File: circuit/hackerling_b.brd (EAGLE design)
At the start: 82.5 x 67.4 mm, 45 parts, among them IC1 MCP23017SP, IC2 MCP2300X/P, IC3 MIC5219BM5, SW2 SWITCH_B13EH, U1 MMA8452Q, U2 LCD_16X2, U3 ARDUINOR3-BPLACE, U4 ACCELEROMETER, U5 PCA9306, U6 ACCELEROMETER, U7 POT, U8 SML_POT

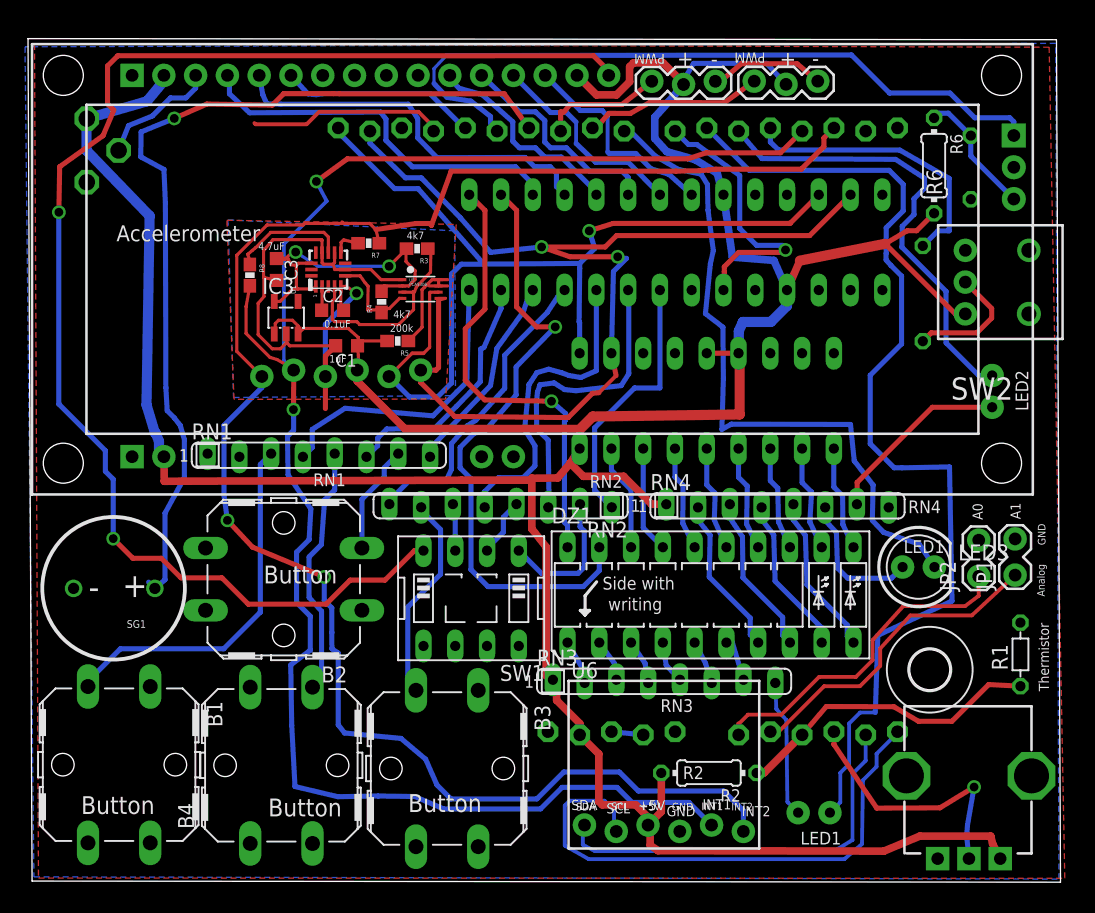
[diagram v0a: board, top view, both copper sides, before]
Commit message: changes made for version 1.2. ordered boards.
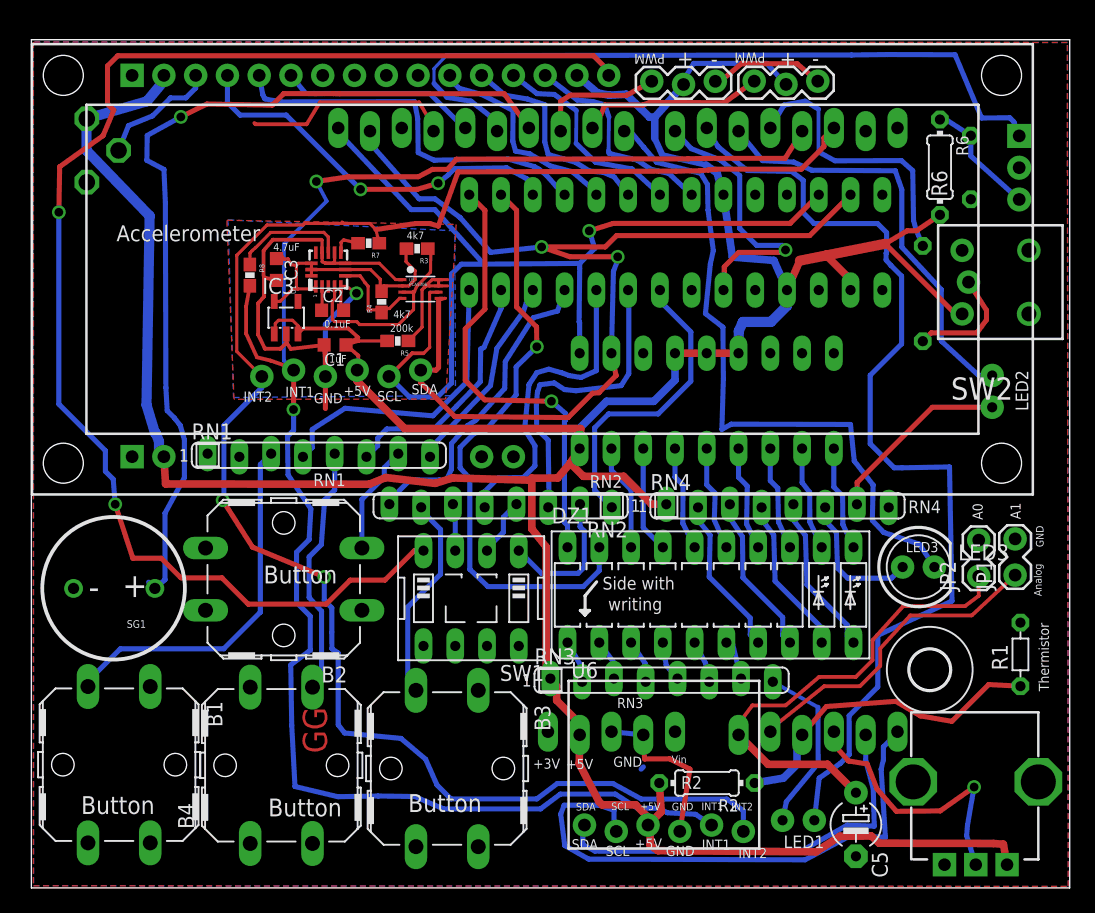
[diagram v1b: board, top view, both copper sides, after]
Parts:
- added C5: (no value), rcl:E5-4
- added U$2: HS-LOGOSMALL, hackerscouts:HS-LOGO-SM
- C4: device rcl:C050-050X075 -> hackerscouts:CAP_050X075
- moved LED1 1.39 mm to (61.3, 4.91)
- moved C1 0.92 mm to (24.3, 42.9)
- moved R2 0.82 mm to (54.0, 7.88)
- moved U7 0.73 mm to (75.5, 7.66)
- moved R6 0.49 mm to (72.6, 57.1)
- moved IR1 0.43 mm to (79.0, 57.1)
- moved RN3 0.22 mm to (50.4, 16.1)
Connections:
- net DIP1 renamed DIP4
- net DIPR1 renamed DIPR4
- net 3.3V: now also U1.15, U1.16, U1.7
- net DIP2: now also RN2.6, SW1.3; no longer RN2.4, SW1.2
- net DIP3: now also RN2.4, SW1.2; no longer RN2.6, SW1.3
- net DIPR2: now also IC1.24, RN2.5; no longer IC1.23, RN2.3
- net DIPR3: now also IC1.23, RN2.3; no longer IC1.24, RN2.5
- net GND: now also C5.-, U1.8; no longer IC1.16, IC2.4, U1.7
- net N$26: now also C5.+
- net VCC: now also IC1.16, IC2.4
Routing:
- net GND: track 75.1 -> 86.9 mm
- net N$26: track 26.8 -> 38.1 mm
- net 3.3V: track 26.6 -> 22.9 mm, vias 2 -> 0
- net DIPR4: track 21.3 -> 24.5 mm
- net N$32: track 11.0 -> 14.1 mm
- net IR_OUT2: track 36.4 -> 33.9 mm
- net BARGRAPH1: track 49.6 -> 47.5 mm
- net IR_OUT1: track 81.2 -> 79.1 mm
- net TEMP: track 24.9 -> 26.5 mm
- net IR_IN: track 58.1 -> 59.5 mm
- net A_INT2: track 138.9 -> 137.6 mm
- net DIP3: track 3.79 -> 4.69 mm
- net DIP2: track 4.69 -> 3.79 mm
- net N$15: track 72.7 -> 71.9 mm
- net SDA: track 88.8 -> 87.9 mm
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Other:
- board size 82.5 x 67.4 mm -> 83 x 67.8 mm
- board text added: "+3V"
- board text added: "28"
- board text added: "6mm away"
- board text added: "Before installing LCD Run all test programs"
- board text added: "GG"
- board text added: "Install Arduino headers on the other side"
- board text added: "LCD"
- board text added: "LED3"
- board text added: "Vin"
- board text removed: "1/4 inch away"
- board text removed: "Install Arduino headers, pointing down."

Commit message: adding version 1.3 schematics
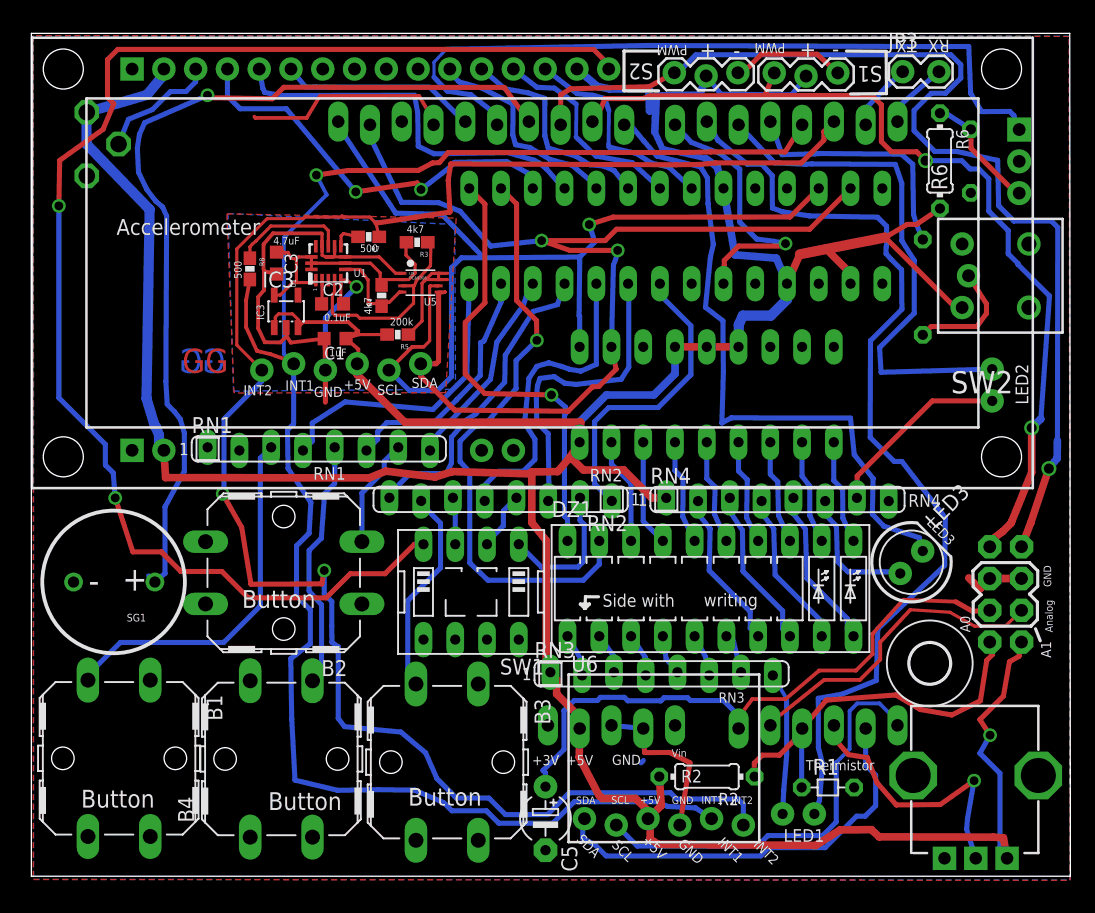
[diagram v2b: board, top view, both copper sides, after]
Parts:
- removed JP1, JP2: (no value), SparkFun:1X02_LOCK
- removed SERVO2: (no value), SparkFun:1X03_LOCK
- removed U$2: HS-LOGOSMALL, hackerscouts:HS-LOGO-SM
- added HACKERSCOUTSLOGO: HS-LOGO, hackerscouts:HS-LOGO-SM-NOTEXT
- added JP3: (no value), SparkFun:1X02_LOCK
- added SERVO: (no value), SparkFun:1X03_LOCK
- added U$1: M04X2, SparkFun:2X4
- SERVO1: value (none) -> SERVO
- moved C5 24.8 mm to (41.1, 5.05)
- moved R1 18.7 mm to (63.7, 7.53), turned to 0 degrees
- moved SERVO1 1.73 mm to (59.4, 64.5)
- moved LED3 0.68 mm to (70.4, 25.5), turned to 45 degrees
- moved C1 0.51 mm to (24.3, 43.4)
- moved C2 0.51 mm to (24.1, 46.2)
- moved IC2 0.51 mm to (54.0, 38.9)
- moved IC3 0.51 mm to (20.4, 45.6)
- moved IR1 0.51 mm to (79.0, 57.6)
- moved LED2 0.51 mm to (76.8, 39.7)
- moved R4 0.51 mm to (28.0, 46.9)
- moved R5 0.51 mm to (29.3, 43.7)
- moved R6 0.51 mm to (72.6, 57.6)
- moved R7 0.51 mm to (27.0, 51.5)
- moved R8 0.51 mm to (17.5, 49.0)
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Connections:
- new net RX: JP3.2, U3.D0
- new net TX: JP3.1, U3.D1
- net GND: now also SERVO.3, U$1.5, U$1.6; no longer JP1.2, JP2.2, SERVO2.3
- net N$24: now also U$1.4; no longer JP1.1
- net N$26: now also U$1.3; no longer JP2.1
- net SVO1: now also U$1.7
- net SVO2: now also SERVO.1, U$1.8; no longer SERVO2.1
- net TEMP: now also U$1.1
- net VCC: now also SERVO.2, U$1.2; no longer SERVO2.2
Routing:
- net SVO2: track 10.1 -> 85.9 mm, vias 0 -> 1
- net SVO1: track 15.2 -> 72.8 mm, vias 0 -> 2
- net VCC: track 284.6 -> 308.8 mm, vias 0 -> 1
- net N$26: track 38.1 -> 49.2 mm
- net SCL1: track 44.4 -> 33.4 mm
- net IR_OUT2: track 33.9 -> 40.9 mm
- net RX: track 0.00 -> 5.51 mm
- net TX: track 0.00 -> 5.47 mm
- net A_INT2: track 137.6 -> 143.0 mm
- net TEMP: track 26.5 -> 31.8 mm
- net GND: track 86.9 -> 91.9 mm
- net IR_OUT1: track 79.1 -> 76.3 mm
- net N$32: track 14.1 -> 11.4 mm
- net SWITCHR: track 22.7 -> 20.0 mm
- net N$10: track 31.2 -> 32.5 mm
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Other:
- board size 83 x 67.8 mm -> 83.1 x 67.4 mm
- board text added: "1.3"
- board text added: "19 & 20"
- board text added: "500"
- board text added: "Hsync"
- board text added: "IC3"
- board text added: "Place MCP23008 here."
- board text added: "Put Your Initials Here"
- board text added: "RX"
- board text added: "S1"
- board text added: "S2"
- board text added: "TX"
- board text added: "U1"
- board text added: "U5"
- board text added: "VGA"
- board text added: "Vsync"
- board text added: "arrow goes here"
- board text added: "blue"
- board text added: "circuit.hackersource.net"
- board text added: "gnd"
- board text added: "grn"
- board text added: "power"
- board text added: "red"
- board text added: "www.hackersource.net"
- board text removed: "1.2"
- board text removed: "19 & 21"
- board text removed: "Bussed array"
- board text removed: "Here"
- board text removed: "Initials"
- board text removed: "Install 4 buttons"
- board text removed: "Place MCP2300 here."
- board text removed: "Put Your"
- board text removed: "arrow"
- board text removed: "circuit.hacker-scouts.org"
- board text removed: "goes"
- board text removed: "www.hacker-scouts.org"
